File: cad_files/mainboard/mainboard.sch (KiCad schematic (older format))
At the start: 58 parts, among them P101 CONN_01X05, P102 CONN_01X02, P103 CONN_01X02, P104 CONN_01X02, P105 CONN_01X03, P106 CONN_01X02, P107 CONN_01X02, P108 CONN_01X02, P109 CONN_01X05, Q101 BC182, Q102 BC182, Q103 BC182, Q104 BC182, Q105 BD137, Q106 BD137, Q107 BD137, Q108 BD137, U101 7805, U102 4N25, U103 4N25, U104 4N25, U105 4N25, U105-JP101 CONN_01X16, U105-JP102 CONN_01X12

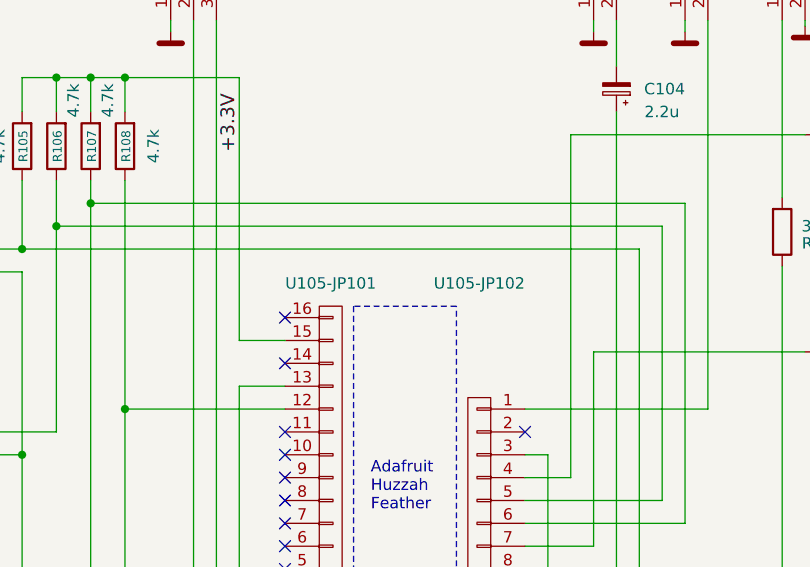
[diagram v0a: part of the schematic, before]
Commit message: 201031
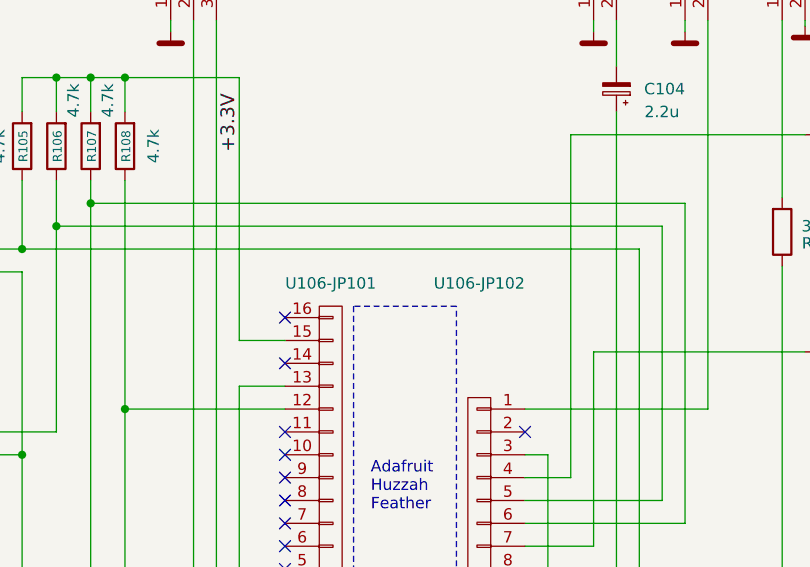
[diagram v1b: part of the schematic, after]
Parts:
- renumbered U105-JP101 to U106-JP101, U105-JP102 to U106-JP102
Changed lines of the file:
@@
 	6075 2475 5625 2475
 $Comp
-L CONN_01X16 U105-JP101
+L CONN_01X16 U106-JP101
 U 1 1 5F19AC96
 P 5525 3275
-F 0 "U105-JP101" H 5525 2375 50  0000 C CNN
+F 0 "U106-JP101" H 5525 2375 50  0000 C CNN
 F 1 "CONN_01X16" V 5625 3275 50  0001 C CNN
 F 2 "Socket_Strips:Socket_Strip_Straight_1x16" H 5525 3275 50  0001 C CNN
@@
 $EndComp
 $Comp
-L CONN_01X12 U105-JP102
+L CONN_01X12 U106-JP102
 U 1 1 5F19AC49
 P 6175 3475
-F 0 "U105-JP102" H 6175 4575 50  0000 C CNN
+F 0 "U106-JP102" H 6175 4575 50  0000 C CNN
 F 1 "CONN_01X12" V 6275 3475 50  0001 C CNN
 F 2 "Socket_Strips:Socket_Strip_Straight_1x12" H 6175 3475 50  0001 C CNN

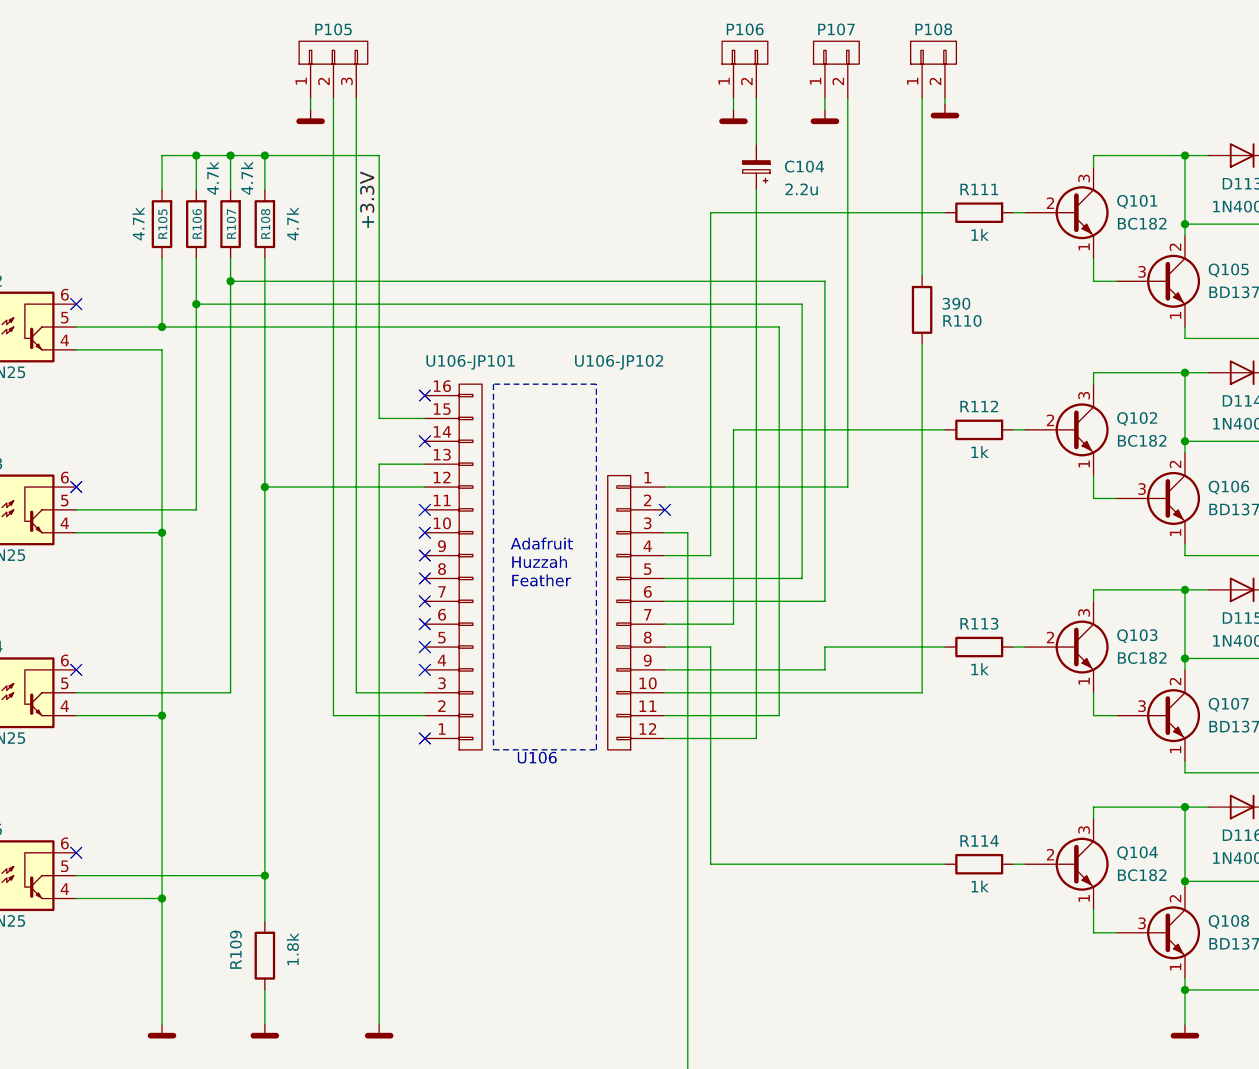
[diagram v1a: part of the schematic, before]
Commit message: 201101
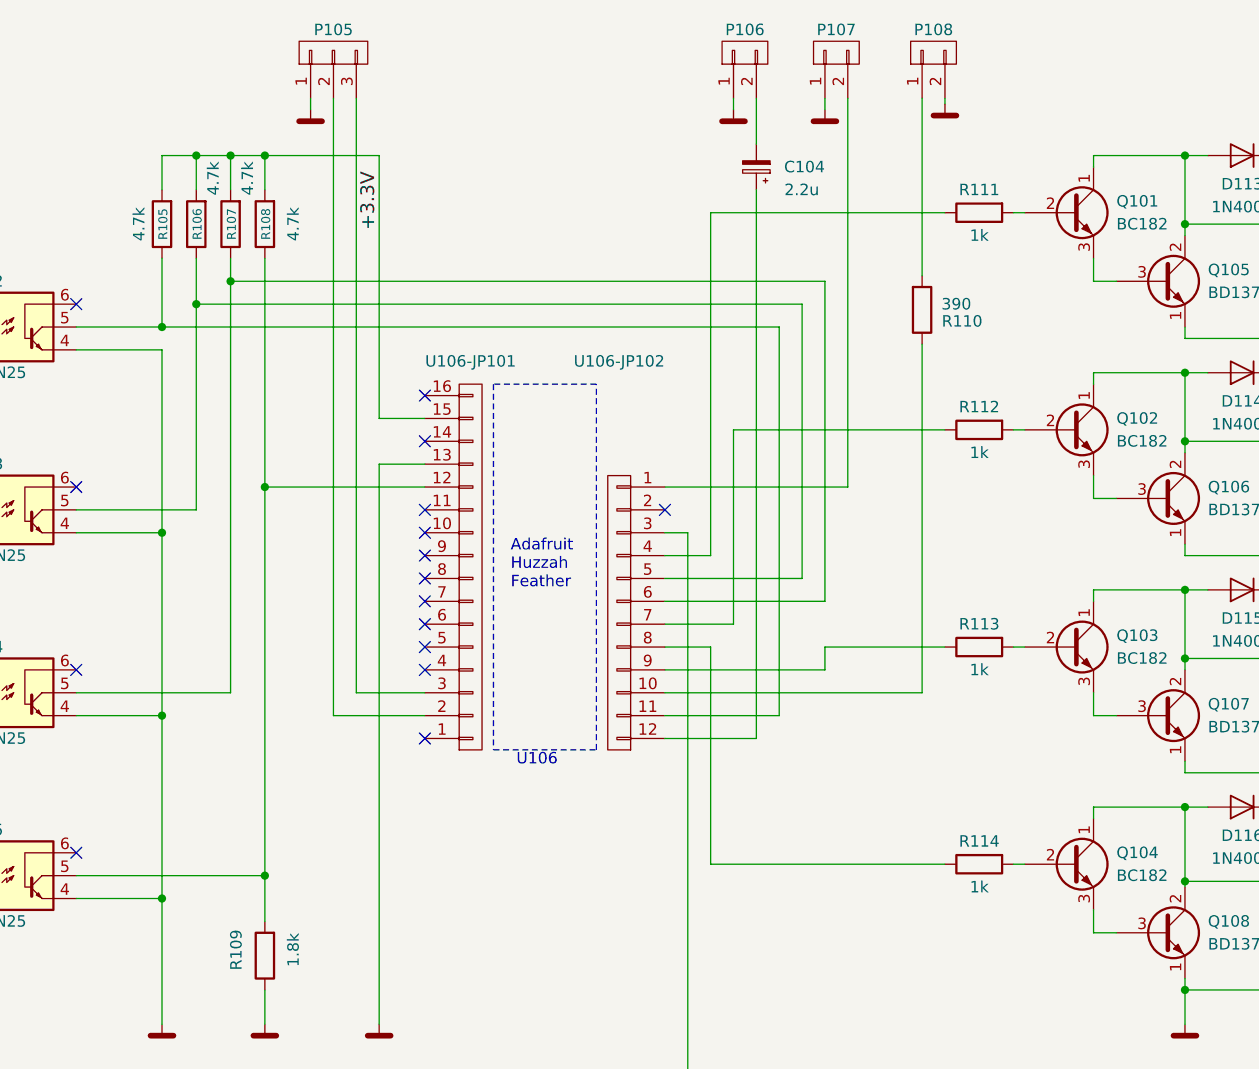
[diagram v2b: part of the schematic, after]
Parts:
- removed Q101, Q102, Q103, Q104: BC182, TO_SOT_Packages_THT:TO-92_Inline_Narrow_Oval, symbol Q_NPN_EBC
- added Q101, Q102, Q103, Q104: BC182, TO_SOT_Packages_THT:TO-92_Molded_Narrow, symbol Q_NPN_CBE
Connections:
- net at R111.2: now also Q101.2 (B)
- net at D115.2 (A), P109.4 (P4), Q107.2 (C): now also Q103.1 (C)
- net at Q107.3 (B): now also Q103.3 (E)
- net at D116.2 (A), P109.5 (P5), Q108.2 (C): now also Q104.1 (C)
- net at Q108.3 (B): now also Q104.3 (E)
- net at D114.2 (A), P109.3 (P3), Q106.2 (C): now also Q102.1 (C)
- net at Q106.3 (B): now also Q102.3 (E)
- net at D113.2 (A), P109.2 (P2), Q105.2 (C): now also Q101.1 (C)
- net at Q105.3 (B): now also Q101.3 (E)
- net at R112.2: now also Q102.2 (B)
- net at R113.2: now also Q103.2 (B)
- net at R114.2: now also Q104.2 (B)
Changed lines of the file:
@@
 	4625 1475 4625 1625
 Wire Wire Line
-	4175 1475 5125 1475
+	5125 1475 4175 1475
 Wire Wire Line
 	4175 1475 4175 1625
@@
 	5125 2825 5125 5275
 $Comp
-L pzs_others:0V #PWR06
+L pzs_others:0V #PWR04
 U 1 1 5F1E7647
 P 4625 5275
-F 0 "#PWR06" H 4625 5025 50  0001 C CNN
+F 0 "#PWR04" H 4625 5025 50  0001 C CNN
 F 1 "0V" H 4625 5125 50  0001 C CNN
 F 2 "" H 4625 5275 50  0000 C CNN
@@
 $EndComp
 $Comp
-L pzs_others:0V #PWR04
+L pzs_others:0V #PWR05
 U 1 1 5F19FE91
 P 4825 1275
-F 0 "#PWR04" H 4825 1025 50  0001 C CNN
+F 0 "#PWR05" H 4825 1025 50  0001 C CNN
 F 1 "0V" H 4825 1125 50  0001 C CNN
 F 2 "" H 4825 1275 50  0000 C CNN
@@
 NoConn ~ 3800 2125
 $Comp
-L pzs_others:0V #PWR03
+L pzs_others:0V #PWR06
 U 1 1 5F1AA249
 P 4175 5275
-F 0 "#PWR03" H 4175 5025 50  0001 C CNN
+F 0 "#PWR06" H 4175 5025 50  0001 C CNN
 F 1 "0V" H 4175 5125 50  0001 C CNN
 F 2 "" H 4175 5275 50  0000 C CNN
@@
 NoConn ~ 5325 2525
 $Comp
-L pzs_others:0V #PWR01
+L pzs_others:0V #PWR07
 U 1 1 5EEE442D
 P 5125 5275
-F 0 "#PWR01" H 5125 5025 50  0001 C CNN
+F 0 "#PWR07" H 5125 5025 50  0001 C CNN
 F 1 "0V" H 5125 5125 50  0001 C CNN
 F 2 "" H 5125 5275 50  0000 C CNN
@@
 	1625 5525 2675 5525
 $Comp
-L pzs_others:0V #PWR010
+L pzs_others:0V #PWR08
 U 1 1 5F9BD0C0
 P 2675 5525
-F 0 "#PWR010" H 2675 5275 50  0001 C CNN
+F 0 "#PWR08" H 2675 5275 50  0001 C CNN
 F 1 "0V" H 2675 5375 50  0001 C CNN
 F 2 "" H 2675 5525 50  0000 C CNN
@@
 $EndComp
 $Comp
-L pzs_others:0V #PWR08
+L pzs_others:0V #PWR010
 U 1 1 5F7F7EA1
 P 2675 6375
-F 0 "#PWR08" H 2675 6125 50  0001 C CNN
+F 0 "#PWR010" H 2675 6125 50  0001 C CNN
 F 1 "0V" H 2675 6225 50  0001 C CNN
 F 2 "" H 2675 6375 50  0000 C CNN
@@
 	8650 5075 8650 5275
 $Comp
-L Q_NPN_EBC Q104
-U 1 1 5F1A19FD
-P 8150 4575
-F 0 "Q104" H 8350 4625 50  0000 L CNN
-F 1 "BC182" H 8350 4525 50  0000 L CNN
-F 2 "TO_SOT_Packages_THT:TO-92_Inline_Narrow_Oval" H 8350 4675 50  0001 C CNN
-F 3 "" H 8150 4575 50  0000 C CNN
-	1    8150 4575
-	1    0    0    -1
-$EndComp
-$Comp
-L Q_NPN_EBC Q103
-U 1 1 5F1A1931
-P 8150 3625
-F 0 "Q103" H 8350 3675 50  0000 L CNN
-F 1 "BC182" H 8350 3575 50  0000 L CNN
-F 2 "TO_SOT_Packages_THT:TO-92_Inline_Narrow_Oval" H 8350 3725 50  0001 C CNN
-F 3 "" H 8150 3625 50  0000 C CNN
-	1    8150 3625
-	1    0    0    -1
-$EndComp
-$Comp
-L Q_NPN_EBC Q102
-U 1 1 5F1A185C
-P 8150 2675
-F 0 "Q102" H 8350 2725 50  0000 L CNN
-F 1 "BC182" H 8350 2625 50  0000 L CNN
-F 2 "TO_SOT_Packages_THT:TO-92_Inline_Narrow_Oval" H 8350 2775 50  0001 C CNN
-F 3 "" H 8150 2675 50  0000 C CNN
-	1    8150 2675
-	1    0    0    -1
-$EndComp
-$Comp
-L Q_NPN_EBC Q101
-U 1 1 5F1A151F
-P 8150 1725
-F 0 "Q101" H 8350 1775 50  0000 L CNN
-F 1 "BC182" H 8350 1675 50  0000 L CNN
-F 2 "TO_SOT_Packages_THT:TO-92_Inline_Narrow_Oval" H 8350 1825 50  0001 C CNN
-F 3 "" H 8150 1725 50  0000 C CNN
-	1    8150 1725
-	1    0    0    -1
-$EndComp
-$Comp
 L Q_NPN_ECB Q105
 U 1 1 5F1A10F1
@@
 $EndComp
 $Comp
-L pzs_others:0V #PWR02
+L pzs_others:0V #PWR011
 U 1 1 5EF79B48
 P 8650 5275
-F 0 "#PWR02" H 8650 5025 50  0001 C CNN
+F 0 "#PWR011" H 8650 5025 50  0001 C CNN
 F 1 "0V" H 8650 5125 50  0001 C CNN
 F 2 "" H 8650 5275 50  0000 C CNN
@@
 	1    0    0    -1
 $EndComp
+$Comp
+L Q_NPN_CBE Q101
+U 1 1 5F9EAEA4
+P 8150 1725
+F 0 "Q101" H 8350 1775 50  0000 L CNN
+F 1 "BC182" H 8350 1675 50  0000 L CNN
+F 2 "TO_SOT_Packages_THT:TO-92_Molded_Narrow" H 8350 1825 50  0001 C CNN
+F 3 "" H 8150 1725 50  0000 C CNN
+	1    8150 1725
+	1    0    0    -1
+$EndComp
+$Comp
+L Q_NPN_CBE Q102
+U 1 1 5F9EB64D
+P 8150 2675
+F 0 "Q102" H 8350 2725 50  0000 L CNN
+F 1 "BC182" H 8350 2625 50  0000 L CNN
+F 2 "TO_SOT_Packages_THT:TO-92_Molded_Narrow" H 8350 2775 50  0001 C CNN
+F 3 "" H 8150 2675 50  0000 C CNN
+	1    8150 2675
+	1    0    0    -1
+$EndComp
+$Comp
+L Q_NPN_CBE Q103
+U 1 1 5F9EB737
+P 8150 3625
+F 0 "Q103" H 8350 3675 50  0000 L CNN
+F 1 "BC182" H 8350 3575 50  0000 L CNN
+F 2 "TO_SOT_Packages_THT:TO-92_Molded_Narrow" H 8350 3725 50  0001 C CNN
+F 3 "" H 8150 3625 50  0000 C CNN
+	1    8150 3625
+	1    0    0    -1
+$EndComp
+$Comp
+L Q_NPN_CBE Q104
+U 1 1 5F9EB816
+P 8150 4575
+F 0 "Q104" H 8350 4625 50  0000 L CNN
+F 1 "BC182" H 8350 4525 50  0000 L CNN
+F 2 "TO_SOT_Packages_THT:TO-92_Molded_Narrow" H 8350 4675 50  0001 C CNN
+F 3 "" H 8150 4575 50  0000 C CNN
+	1    8150 4575
+	1    0    0    -1
+$EndComp
